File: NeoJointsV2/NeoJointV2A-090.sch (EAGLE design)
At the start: 5 parts

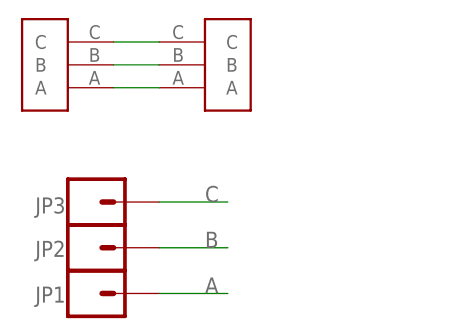
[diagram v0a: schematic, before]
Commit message: update neojointv2a
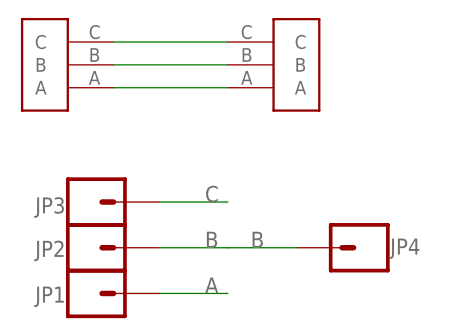
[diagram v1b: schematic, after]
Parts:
- added JP4: (no value), SparkFun-Connectors:M01PTH
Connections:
- net B: now also JP4.1
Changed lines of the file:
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@@
 <part name="U$1" library="todstuff" deviceset="LED_STRIP_3P" device=""/>
 <part name="U$2" library="todstuff" deviceset="LED_STRIP_3P" device=""/>
+<part name="JP4" library="SparkFun-Connectors" deviceset="M01" device="PTH"/>
 </parts>
 <sheets>
@@
 <attribute name="NAME" x="27.686" y="89.408" size="1.778" layer="95" rot="R180"/>
 </instance>
-<instance part="U$1" gate="G$1" x="43.18" y="104.14"/>
+<instance part="U$1" gate="G$1" x="50.8" y="104.14"/>
 <instance part="U$2" gate="G$1" x="27.94" y="104.14" rot="MR0"/>
+<instance part="JP4" gate="G$1" x="60.96" y="83.82" smashed="yes" rot="R180">
+<attribute name="VALUE" x="63.5" y="88.9" size="1.778" layer="96" rot="R180"/>
+<attribute name="NAME" x="63.754" y="83.058" size="1.778" layer="95"/>
+</instance>
 </instances>
 <busses>
@@
 <pinref part="U$1" gate="G$1" pin="A"/>
 <pinref part="U$2" gate="G$1" pin="A"/>
-<wire x1="33.02" y1="101.6" x2="38.1" y2="101.6" width="0.1524" layer="91"/>
-</segment>
-</net>
-<net name="B" class="0">
-<segment>
-<wire x1="38.1" y1="83.82" x2="45.72" y2="83.82" width="0.1524" layer="91"/>
-<label x="43.18" y="83.82" size="1.778" layer="95"/>
-<pinref part="JP2" gate="G$1" pin="1"/>
-</segment>
-<segment>
-<pinref part="U$1" gate="G$1" pin="B"/>
-<pinref part="U$2" gate="G$1" pin="B"/>
-<wire x1="33.02" y1="104.14" x2="38.1" y2="104.14" width="0.1524" layer="91"/>
+<wire x1="33.02" y1="101.6" x2="45.72" y2="101.6" width="0.1524" layer="91"/>
 </segment>
 </net>
@@
 <pinref part="U$1" gate="G$1" pin="C"/>
 <pinref part="U$2" gate="G$1" pin="C"/>
-<wire x1="33.02" y1="106.68" x2="38.1" y2="106.68" width="0.1524" layer="91"/>
+<wire x1="33.02" y1="106.68" x2="45.72" y2="106.68" width="0.1524" layer="91"/>
 </segment>
 </net>
+<net name="B" class="0">
+<segment>
+<pinref part="U$2" gate="G$1" pin="B"/>
+<pinref part="U$1" gate="G$1" pin="B"/>
+<wire x1="33.02" y1="104.14" x2="45.72" y2="104.14" width="0.1524" layer="91"/>
+</segment>
+<segment>
+<pinref part="JP2" gate="G$1" pin="1"/>
+<wire x1="38.1" y1="83.82" x2="45.72" y2="83.82" width="0.1524" layer="91"/>
+<label x="43.18" y="83.82" size="1.778" layer="95"/>
+<pinref part="JP4" gate="G$1" pin="1"/>
+<wire x1="53.34" y1="83.82" x2="48.26" y2="83.82" width="0.1524" layer="91"/>
+<label x="48.26" y="83.82" size="1.778" layer="95"/>
+<wire x1="45.72" y1="83.82" x2="48.26" y2="83.82" width="0.1524" layer="91"/>
+</segment>
+</net>
